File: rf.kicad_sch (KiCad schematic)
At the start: 2 parts, among them U3 RFM95W-868S2

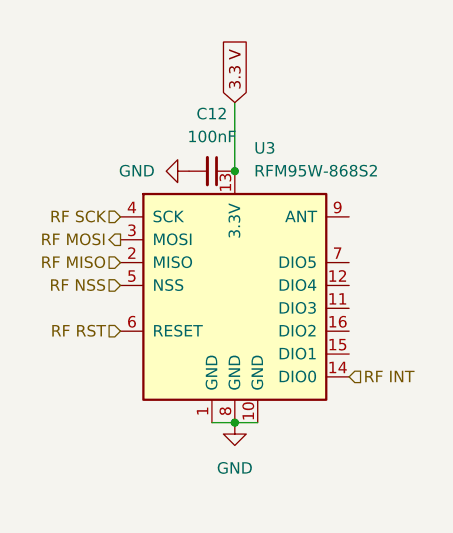
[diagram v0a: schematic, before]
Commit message: Clean up
Minor fixes to mistakes in the schematic
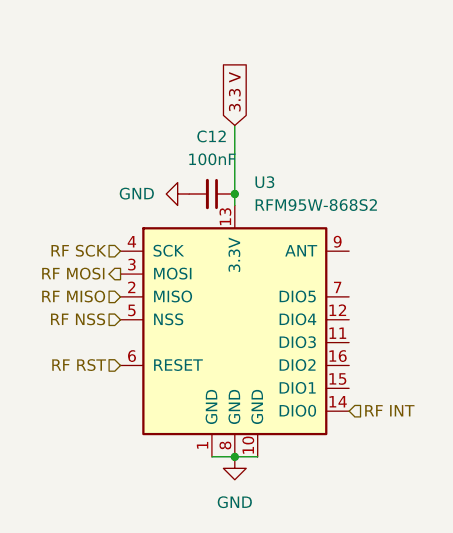
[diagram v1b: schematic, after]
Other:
- moved on the sheet: C12, U3
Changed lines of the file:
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@@
 	(paper "A4")
 	(junction
-		(at 41.91 57.15)
+		(at 41.91 60.96)
 		(diameter 0)
 		(color 0 0 0 0)
 	)
 	(junction
-		(at 41.91 29.21)
+		(at 41.91 31.75)
 		(diameter 0)
 		(color 0 0 0 0)
@@
 	(wire
 		(pts
-			(xy 41.91 21.59) (xy 41.91 29.21)
+			(xy 41.91 24.13) (xy 41.91 31.75)
 		)
 		(stroke
@@
 	(wire
 		(pts
-			(xy 39.37 57.15) (xy 41.91 57.15)
+			(xy 39.37 60.96) (xy 41.91 60.96)
 		)
 		(stroke
@@
 	(wire
 		(pts
-			(xy 41.91 57.15) (xy 44.45 57.15)
+			(xy 41.91 31.75) (xy 41.91 33.02)
 		)
 		(stroke
@@
 		)
 	)
+	(wire
+		(pts
+			(xy 41.91 60.96) (xy 44.45 60.96)
+		)
+		(stroke
+			(width 0)
+			(type default)
+		)
+	)
 	(global_label "3.3 V"
 		(shape input)
-		(at 41.91 21.59 90)
+		(at 41.91 24.13 90)
 		(fields_autoplaced yes)
 		(effects
@@
 		)
 		(property "Intersheetrefs" "${INTERSHEET_REFS}"
-			(at 41.91 13.5248 90)
+			(at 41.91 16.0648 90)
 			(hide yes)
 			(show_name no)
@@
 	(hierarchical_label "RF NSS"
 		(shape input)
-		(at 29.21 41.91 180)
+		(at 29.21 45.72 180)
 		(effects
 			(font
@@
 	(hierarchical_label "RF SCK"
 		(shape input)
-		(at 29.21 34.29 180)
+		(at 29.21 38.1 180)
 		(effects
 			(font
@@
 	(hierarchical_label "RF MISO"
 		(shape input)
-		(at 29.21 39.37 180)
+		(at 29.21 43.18 180)
 		(effects
 			(font
@@
 	(hierarchical_label "RF MOSI"
 		(shape output)
-		(at 29.21 36.83 180)
+		(at 29.21 40.64 180)
 		(effects
 			(font
@@
 	(hierarchical_label "RF INT"
 		(shape input)
-		(at 54.61 52.07 0)
+		(at 54.61 55.88 0)
 		(effects
 			(font
@@
 	(hierarchical_label "RF RST"
 		(shape input)
-		(at 29.21 46.99 180)
+		(at 29.21 50.8 180)
 		(effects
 			(font
@@
 	(symbol
 		(lib_id "Device:C_Small")
-		(at 39.37 29.21 270)
+		(at 39.37 31.75 270)
 		(unit 1)
 		(body_style 1)
@@
 		(fields_autoplaced yes)
 		(property "Reference" "C12"
-			(at 39.3636 22.86 90)
+			(at 39.3636 25.4 90)
 			(show_name no)
 			(do_not_autoplace no)
@@
 		)
 		(property "Value" "100nF"
-			(at 39.3636 25.4 90)
+			(at 39.3636 27.94 90)
 			(show_name no)
 			(do_not_autoplace no)
@@
 		)
 		(property "Footprint" ""
-			(at 39.37 29.21 0)
+			(at 39.37 31.75 0)
 			(hide yes)
 			(show_name no)
@@
 		)
 		(property "Datasheet" ""
-			(at 39.37 29.21 0)
+			(at 39.37 31.75 0)
 			(hide yes)
 			(show_name no)
@@
 		)
 		(property "Description" "Unpolarized capacitor, small symbol"
-			(at 39.37 29.21 0)
+			(at 39.37 31.75 0)
 			(hide yes)
 			(show_name no)
@@
 	(symbol
 		(lib_id "power:GND")
-		(at 41.91 57.15 0)
+		(at 41.91 60.96 0)
 		(unit 1)
 		(body_style 1)
@@
 		(fields_autoplaced yes)
 		(property "Reference" "#PWR011"
-			(at 41.91 63.5 0)
+			(at 41.91 67.31 0)
 			(hide yes)
 			(show_name no)
@@
 		)
 		(property "Value" "GND"
-			(at 41.91 62.23 0)
+			(at 41.91 66.04 0)
 			(show_name no)
 			(do_not_autoplace no)
@@
 		)
 		(property "Footprint" ""
-			(at 41.91 57.15 0)
+			(at 41.91 60.96 0)
 			(hide yes)
 			(show_name no)
@@
 		)
 		(property "Datasheet" ""
-			(at 41.91 57.15 0)
+			(at 41.91 60.96 0)
 			(hide yes)
 			(show_name no)
@@
 		)
 		(property "Description" "Power symbol creates a global label with name \"GND\" , ground"
-			(at 41.91 57.15 0)
+			(at 41.91 60.96 0)
 			(hide yes)
 			(show_name no)
@@
 	(symbol
 		(lib_id "power:GND")
-		(at 36.83 29.21 270)
+		(at 36.83 31.75 270)
 		(unit 1)
 		(body_style 1)
@@
 		(fields_autoplaced yes)
 		(property "Reference" "#PWR017"
-			(at 30.48 29.21 0)
+			(at 30.48 31.75 0)
 			(hide yes)
 			(show_name no)
@@
 		)
 		(property "Value" "GND"
-			(at 33.02 29.2099 90)
+			(at 33.02 31.7499 90)
 			(show_name no)
 			(do_not_autoplace no)
@@
 		)
 		(property "Footprint" ""
-			(at 36.83 29.21 0)
+			(at 36.83 31.75 0)
 			(hide yes)
 			(show_name no)
@@
 		)
 		(property "Datasheet" ""
-			(at 36.83 29.21 0)
+			(at 36.83 31.75 0)
 			(hide yes)
 			(show_name no)
@@
 		)
 		(property "Description" "Power symbol creates a global label with name \"GND\" , ground"
-			(at 36.83 29.21 0)
+			(at 36.83 31.75 0)
 			(hide yes)
 			(show_name no)
@@
 	(symbol
 		(lib_id "RF_Module:RFM95W-868S2")
-		(at 41.91 41.91 0)
+		(at 41.91 45.72 0)
 		(unit 1)
 		(body_style 1)
@@
 		(fields_autoplaced yes)
 		(property "Reference" "U3"
-			(at 44.0533 26.67 0)
+			(at 44.0533 30.48 0)
 			(show_name no)
 			(do_not_autoplace no)
@@
 		)
 		(property "Value" "RFM95W-868S2"
-			(at 44.0533 29.21 0)
+			(at 44.0533 33.02 0)
 			(show_name no)
 			(do_not_autoplace no)
@@
 		)
 		(property "Footprint" ""
-			(at -41.91 0 0)
+			(at -41.91 3.81 0)
 			(hide yes)
 			(show_name no)
@@
 		)
 		(property "Datasheet" "https://www.hoperf.com/data/upload/portal/20181127/5bfcbea20e9ef.pdf"
-			(at -41.91 0 0)
+			(at -41.91 3.81 0)
 			(hide yes)
 			(show_name no)
@@
 		)
 		(property "Description" "Low power long range transceiver module, SPI and parallel interface, 868 MHz, spreading factor 6 to12, bandwidth 7.8 to 500kHz, -111 to -148 dBm, SMD-16, DIP-16"
-			(at 41.91 41.91 0)
-			(hide yes)
-			(show_name no)
+			(at 41.91 45.72 0)
+			(hide yes)
+			(show_name no)
